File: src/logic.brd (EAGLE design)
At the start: 36 x 73.5 mm, 95 parts, among them CON1 CON-4P-TABS-JST_GH-RA, CON11 PINHEAD_1X04-2, CON12 PINHEAD_1X04-2, CON2 PINHEAD_1X04-2.54, CON3 PINHEAD_2X04-PLS-2, CON6 PINHEAD_2X02-PTH-2-MALE, CON7 PINHEAD_2X02-PTH-2-MALE, IC1 STM32F105RCT6, IC10 LM75-TSSOP8, IC101 LM5017, IC11 LM75-TSSOP8, IC2 CAT24C02, IC201 TPS62160QDSGRQ1, IC3 AP2127-3.3, IC5 INA180A2, IC6 LMV331, IC7 ST3232, IC8 LM75-TSSOP8, X1 16MHz

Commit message: Values of the current amp filter  updated
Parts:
- C12: value (none) -> 1000pF
- R13, R18: value 4R7 -> 000
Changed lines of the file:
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@@
 <attribute name="TOLERANCE" value="1%" x="-9.2" y="69.9" size="1.778" layer="27" display="off"/>
 </element>
-<element name="R13" library="rc" library_urn="urn:adsk.eagle:library:2539423" package="R0402" package3d_urn="urn:adsk.eagle:package:2539456/2" value="4R7" x="-8.35" y="71.5" smashed="yes">
+<element name="R13" library="rc" library_urn="urn:adsk.eagle:library:2539423" package="R0402" package3d_urn="urn:adsk.eagle:package:2539456/2" value="000" x="-8.35" y="71.5" smashed="yes">
 <attribute name="AEC-Q" value="" x="-8.35" y="71.5" size="1.778" layer="27" display="off"/>
 <attribute name="DIGIKEY#" value="" x="-8.35" y="71.5" size="1.778" layer="27" display="off"/>
@@
 <attribute name="TOLERANCE" value="1%" x="-8.35" y="71.5" size="1.778" layer="27" display="off"/>
 </element>
-<element name="R18" library="rc" library_urn="urn:adsk.eagle:library:2539423" package="R0402" package3d_urn="urn:adsk.eagle:package:2539456/2" value="4R7" x="-8.35" y="72.6" smashed="yes">
+<element name="R18" library="rc" library_urn="urn:adsk.eagle:library:2539423" package="R0402" package3d_urn="urn:adsk.eagle:package:2539456/2" value="000" x="-8.35" y="72.6" smashed="yes">
 <attribute name="AEC-Q" value="" x="-8.35" y="72.6" size="1.778" layer="27" display="off"/>
 <attribute name="DIGIKEY#" value="" x="-8.35" y="72.6" size="1.778" layer="27" display="off"/>
@@
 <attribute name="TOLERANCE" value="1%" x="-8.35" y="72.6" size="1.778" layer="27" display="off"/>
 </element>
-<element name="C12" library="rc" library_urn="urn:adsk.eagle:library:2539423" package="C0402" package3d_urn="urn:adsk.eagle:package:2539461/2" value="" x="-9.9" y="72.05" smashed="yes" rot="R90">
+<element name="C12" library="rc" library_urn="urn:adsk.eagle:library:2539423" package="C0402" package3d_urn="urn:adsk.eagle:package:2539461/2" value="1000pF" x="-9.9" y="72.05" smashed="yes" rot="R90">
 <attribute name="AEC-Q" value="" x="-9.9" y="72.05" size="1.778" layer="27" rot="R90" display="off"/>
 <attribute name="DIGIKEY#" value="" x="-9.9" y="72.05" size="1.778" layer="27" rot="R90" display="off"/>

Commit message: phase sensing nominals updated
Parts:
- R11, R15, R9: value 5K6 -> 1K5
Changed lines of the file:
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@@
 <attribute name="TOLERANCE" value="1%" x="-3.65" y="56.5" size="1.778" layer="27" rot="R90" display="off"/>
 </element>
-<element name="R15" library="rc" library_urn="urn:adsk.eagle:library:2539423" package="R0402" package3d_urn="urn:adsk.eagle:package:2539456/2" value="5K6" x="-3.45" y="57.25" smashed="yes" rot="R90">
+<element name="R15" library="rc" library_urn="urn:adsk.eagle:library:2539423" package="R0402" package3d_urn="urn:adsk.eagle:package:2539456/2" value="1K5" x="-3.45" y="57.25" smashed="yes" rot="R90">
 <attribute name="AEC-Q" value="" x="-3.45" y="57.25" size="1.778" layer="27" rot="R90" display="off"/>
 <attribute name="DIGIKEY#" value="" x="-0.95" y="57.25" size="1.778" layer="27" rot="R90" display="off"/>
@@
 <attribute name="TOLERANCE" value="1%" x="-1.48223125" y="60.002940625" size="1.778" layer="27" rot="R45" display="off"/>
 </element>
-<element name="R9" library="rc" library_urn="urn:adsk.eagle:library:2539423" package="R0402" package3d_urn="urn:adsk.eagle:package:2539456/2" value="5K6" x="-0.790378125" y="64.173221875" smashed="yes" rot="R135">
+<element name="R9" library="rc" library_urn="urn:adsk.eagle:library:2539423" package="R0402" package3d_urn="urn:adsk.eagle:package:2539456/2" value="1K5" x="-0.790378125" y="64.173221875" smashed="yes" rot="R135">
 <attribute name="AEC-Q" value="" x="-0.790378125" y="64.173221875" size="1.778" layer="27" rot="R135" display="off"/>
 <attribute name="DIGIKEY#" value="" x="0.977384375" y="65.9409875" size="1.778" layer="27" rot="R135" display="off"/>
@@
 <attribute name="TOLERANCE" value="1%" x="-5.62634375" y="68.750609375" size="1.778" layer="27" rot="R225" display="off"/>
 </element>
-<element name="R11" library="rc" library_urn="urn:adsk.eagle:library:2539423" package="R0402" package3d_urn="urn:adsk.eagle:package:2539456/2" value="5K6" x="-3.018196875" y="64.845403125" smashed="yes" rot="R315">
+<element name="R11" library="rc" library_urn="urn:adsk.eagle:library:2539423" package="R0402" package3d_urn="urn:adsk.eagle:package:2539456/2" value="1K5" x="-3.018196875" y="64.845403125" smashed="yes" rot="R315">
 <attribute name="AEC-Q" value="" x="-3.018196875" y="64.845403125" size="1.778" layer="27" rot="R315" display="off"/>
 <attribute name="DIGIKEY#" value="" x="-4.7859625" y="63.0776375" size="1.778" layer="27" rot="R315" display="off"/>

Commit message: Phase sensing filter update
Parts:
- C22, C25, C30: value 1800pF -> 180pF
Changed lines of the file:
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@@
 <attribute name="NAME" x="-5.25" y="53" locked="yes" size="1" layer="25" font="vector" ratio="15" align="center"/>
 </element>
-<element name="C30" library="rc" library_urn="urn:adsk.eagle:library:2539423" package="C0402" package3d_urn="urn:adsk.eagle:package:2539461/2" value="1800pF" x="-4.6" y="57.25" smashed="yes" rot="R90">
+<element name="C30" library="rc" library_urn="urn:adsk.eagle:library:2539423" package="C0402" package3d_urn="urn:adsk.eagle:package:2539461/2" value="180pF" x="-4.6" y="57.25" smashed="yes" rot="R90">
 <attribute name="AEC-Q" value="" x="-4.6" y="57.25" size="1.778" layer="27" rot="R90" display="off"/>
 <attribute name="DIGIKEY#" value="" x="-9.6" y="57.25" size="1.778" layer="27" rot="R90" display="off"/>
@@
 <attribute name="TOLERANCE" value="1%" x="-0.95" y="57.25" size="1.778" layer="27" rot="R90" display="off"/>
 </element>
-<element name="C22" library="rc" library_urn="urn:adsk.eagle:library:2539423" package="C0402" package3d_urn="urn:adsk.eagle:package:2539461/2" value="1800pF" x="-1.568196875" y="63.395403125" smashed="yes" rot="R135">
+<element name="C22" library="rc" library_urn="urn:adsk.eagle:library:2539423" package="C0402" package3d_urn="urn:adsk.eagle:package:2539461/2" value="180pF" x="-1.568196875" y="63.395403125" smashed="yes" rot="R135">
 <attribute name="AEC-Q" value="" x="-1.568196875" y="63.395403125" size="1.778" layer="27" rot="R135" display="off"/>
 <attribute name="DIGIKEY#" value="" x="-5.10373125" y="59.859871875" size="1.778" layer="27" rot="R135" display="off"/>
@@
 <attribute name="TOLERANCE" value="1%" x="0.977384375" y="65.9409875" size="1.778" layer="27" rot="R135" display="off"/>
 </element>
-<element name="C25" library="rc" library_urn="urn:adsk.eagle:library:2539423" package="C0402" package3d_urn="urn:adsk.eagle:package:2539461/2" value="1800pF" x="-2.240378125" y="65.623221875" smashed="yes" rot="R315">
+<element name="C25" library="rc" library_urn="urn:adsk.eagle:library:2539423" package="C0402" package3d_urn="urn:adsk.eagle:package:2539461/2" value="180pF" x="-2.240378125" y="65.623221875" smashed="yes" rot="R315">
 <attribute name="AEC-Q" value="" x="-2.240378125" y="65.623221875" size="1.778" layer="27" rot="R315" display="off"/>
 <attribute name="DIGIKEY#" value="" x="1.295153125" y="69.15875625" size="1.778" layer="27" rot="R315" display="off"/>

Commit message: BEMF filter update
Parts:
- C22, C25, C30: value 180pF -> 5600pF
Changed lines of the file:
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@@
 <attribute name="NAME" x="-5.25" y="53" locked="yes" size="1" layer="25" font="vector" ratio="15" align="center"/>
 </element>
-<element name="C30" library="rc" library_urn="urn:adsk.eagle:library:2539423" package="C0402" package3d_urn="urn:adsk.eagle:package:2539461/2" value="180pF" x="-4.6" y="57.25" smashed="yes" rot="R90">
+<element name="C30" library="rc" library_urn="urn:adsk.eagle:library:2539423" package="C0402" package3d_urn="urn:adsk.eagle:package:2539461/2" value="5600pF" x="-4.6" y="57.25" smashed="yes" rot="R90">
 <attribute name="AEC-Q" value="" x="-4.6" y="57.25" size="1.778" layer="27" rot="R90" display="off"/>
 <attribute name="DIGIKEY#" value="" x="-9.6" y="57.25" size="1.778" layer="27" rot="R90" display="off"/>
@@
 <attribute name="TOLERANCE" value="1%" x="-0.95" y="57.25" size="1.778" layer="27" rot="R90" display="off"/>
 </element>
-<element name="C22" library="rc" library_urn="urn:adsk.eagle:library:2539423" package="C0402" package3d_urn="urn:adsk.eagle:package:2539461/2" value="180pF" x="-1.568196875" y="63.395403125" smashed="yes" rot="R135">
+<element name="C22" library="rc" library_urn="urn:adsk.eagle:library:2539423" package="C0402" package3d_urn="urn:adsk.eagle:package:2539461/2" value="5600pF" x="-1.568196875" y="63.395403125" smashed="yes" rot="R135">
 <attribute name="AEC-Q" value="" x="-1.568196875" y="63.395403125" size="1.778" layer="27" rot="R135" display="off"/>
 <attribute name="DIGIKEY#" value="" x="-5.10373125" y="59.859871875" size="1.778" layer="27" rot="R135" display="off"/>
@@
 <attribute name="TOLERANCE" value="1%" x="0.977384375" y="65.9409875" size="1.778" layer="27" rot="R135" display="off"/>
 </element>
-<element name="C25" library="rc" library_urn="urn:adsk.eagle:library:2539423" package="C0402" package3d_urn="urn:adsk.eagle:package:2539461/2" value="180pF" x="-2.240378125" y="65.623221875" smashed="yes" rot="R315">
+<element name="C25" library="rc" library_urn="urn:adsk.eagle:library:2539423" package="C0402" package3d_urn="urn:adsk.eagle:package:2539461/2" value="5600pF" x="-2.240378125" y="65.623221875" smashed="yes" rot="R315">
 <attribute name="AEC-Q" value="" x="-2.240378125" y="65.623221875" size="1.778" layer="27" rot="R315" display="off"/>
 <attribute name="DIGIKEY#" value="" x="1.295153125" y="69.15875625" size="1.778" layer="27" rot="R315" display="off"/>

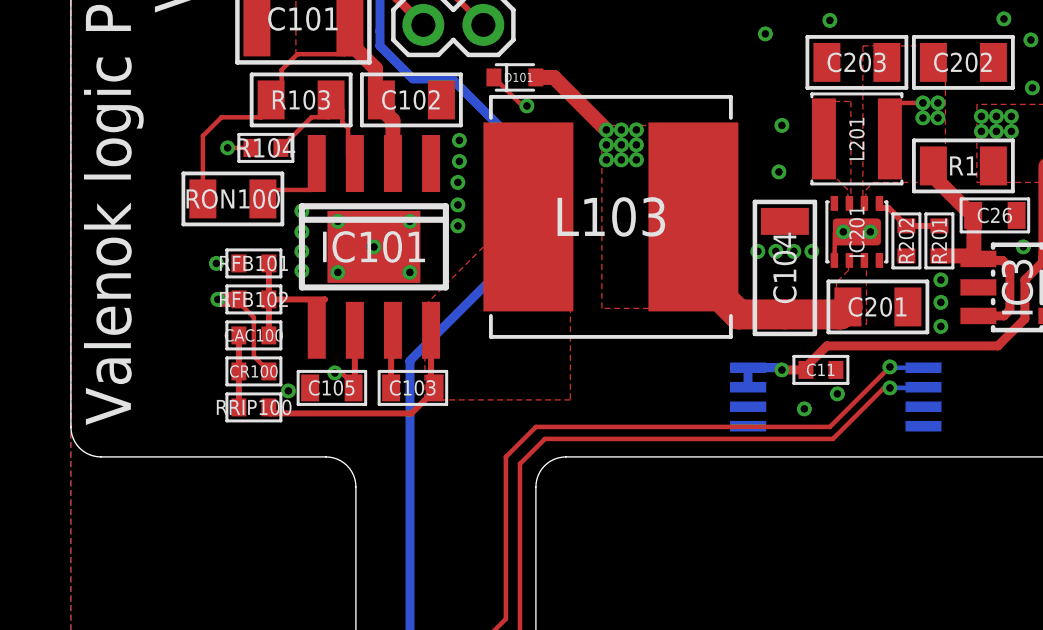
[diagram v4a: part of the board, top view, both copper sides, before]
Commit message: massibe attribute updates everywhere
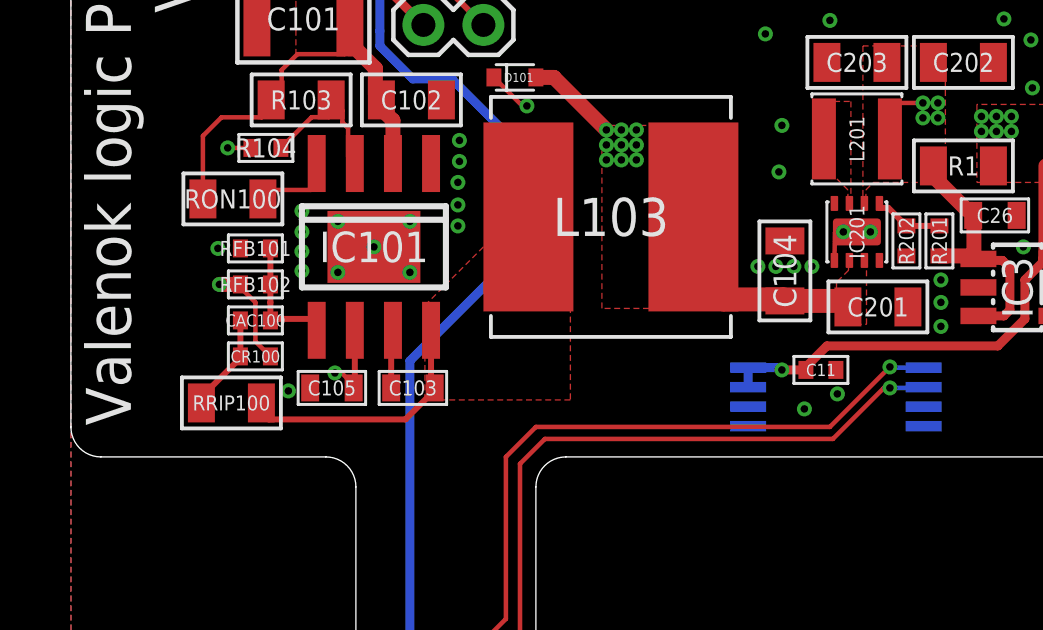
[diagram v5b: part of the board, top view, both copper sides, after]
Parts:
- C10: device C_digikey:C0402 -> rc:C0402
- C101: value 2.2uF -> 2.2µF
- C104: device rc:C1206 -> rc:C0805
- C105: value 1uf -> 1µF
- C15: value 2200pF -> 5600pF
- R5: value 60K -> 110K
- R6: value 2K -> 3K3
- RRIP100: device rc:R0402 -> rc:R0805
- moved RRIP100 0.76 mm to (-12.7, 36.8)
- moved CAC100 0.50 mm to (-11.8, 39.5)
- moved CR100 0.50 mm to (-11.8, 38.4)
- moved RFB101 0.50 mm to (-11.8, 42.0)
- moved RFB102 0.50 mm to (-11.8, 40.8)
- moved C104 0.10 mm to (5.80, 41.2)
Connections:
- net GND: now also C104.1; no longer C104.P$1
- net VDD_12V: now also C104.2; no longer C104.P$2
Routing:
- net HV_DC-DC(LM5017):N$14: track 5.41 -> 4.35 mm
- net HV_DC-DC(LM5017):N$3: track 2.40 -> 3.29 mm
- net HV_DC-DC(LM5017):N$2: track 8.06 -> 8.89 mm
